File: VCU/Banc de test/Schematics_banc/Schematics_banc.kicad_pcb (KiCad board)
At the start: 2 copper layers, 152.5 x 127 mm, 165 parts, among them IC1 TPS7B8633QDDARQ1, IC2 ATA6561-GBQW-N, IC3 TPS7B8633QDDARQ1, J1 2P Angle 171857-4002, J10 2P Droit 2-11-2022, J11 4P Droit 22-11-2042, J12 DM3AT-SF-PEJM5_40_, J2 2P Droit 2-11-2022, J3 4P Droit 22-11-2042, J4 4P Droit 22-11-2042, J5 6P Droit 22-11-2062, J6 6P Droit 22-11-2062, J7 10-97-7086, J8 10-97-7086, J9 2P Droit 2-11-2022, Q1 MMBF170, Q10 SI2337DS-T1-BE3, Q11 SI2337DS-T1-BE3, Q12 SI2337DS-T1-BE3, Q13 SI2337DS-T1-BE3, Q14 SI2337DS-T1-BE3, Q15 SI2337DS-T1-BE3, Q16 SI2337DS-T1-BE3, Q17 BSS138, Q18 BSS138, Q19 BSS138, Q2 MMBF170, Q20 BSS138, Q3 MMBF170, Q4 MMBF170, Q5 MMBF170, Q6 MMBF170, Q7 MMBF170, Q8 MMBF170, Q9 SI2337DS-T1-BE3

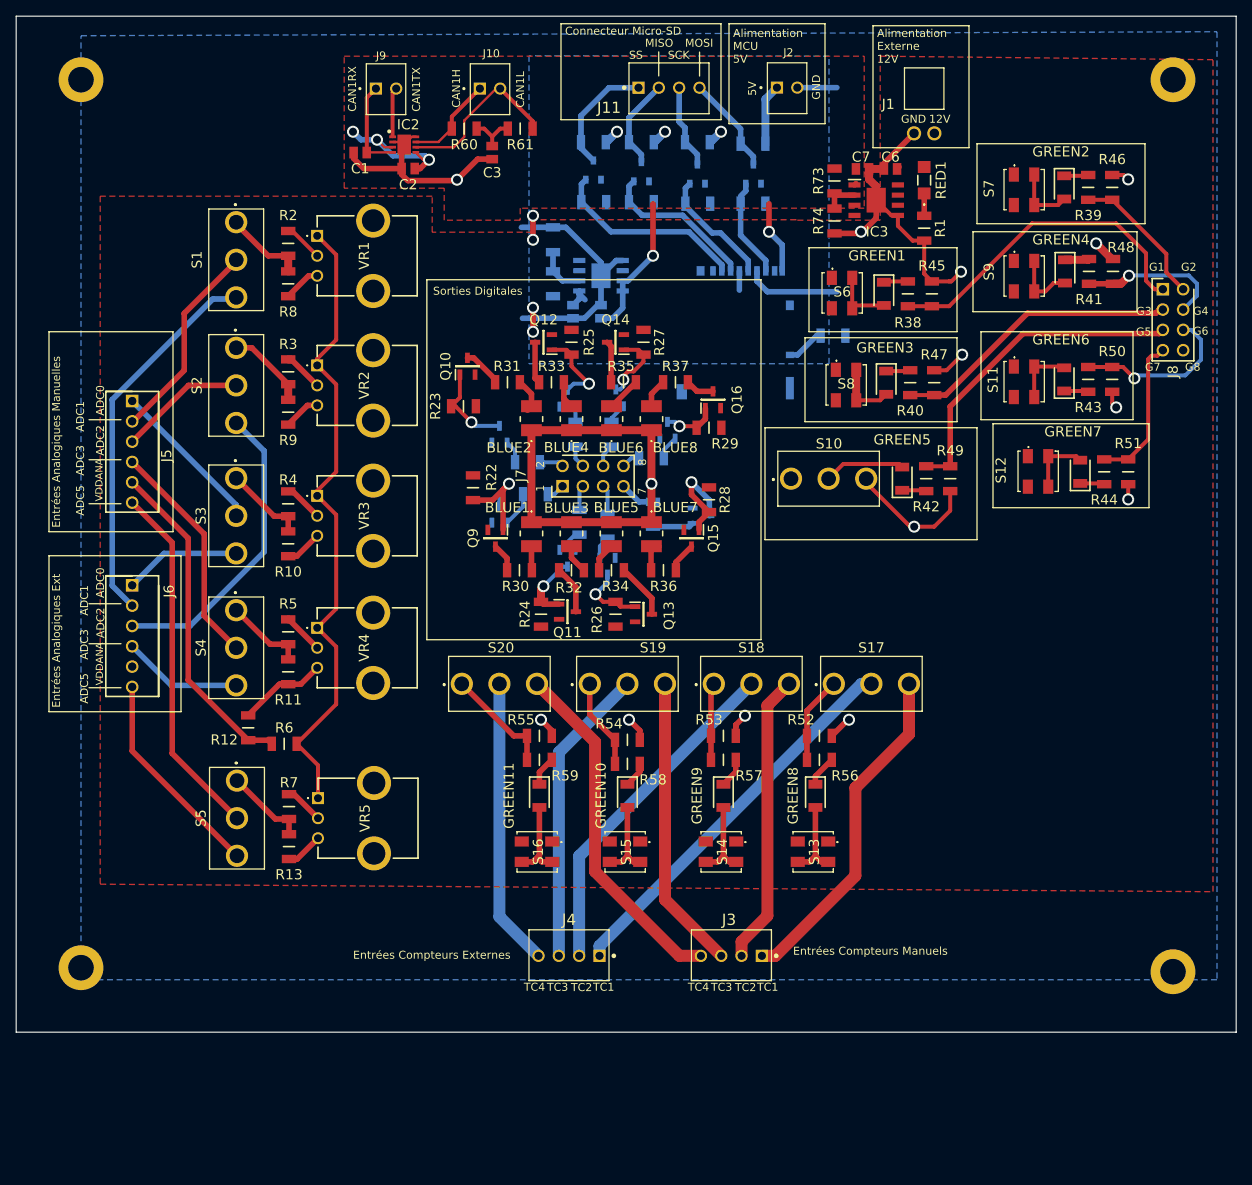
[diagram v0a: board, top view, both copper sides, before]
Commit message: Routage Final
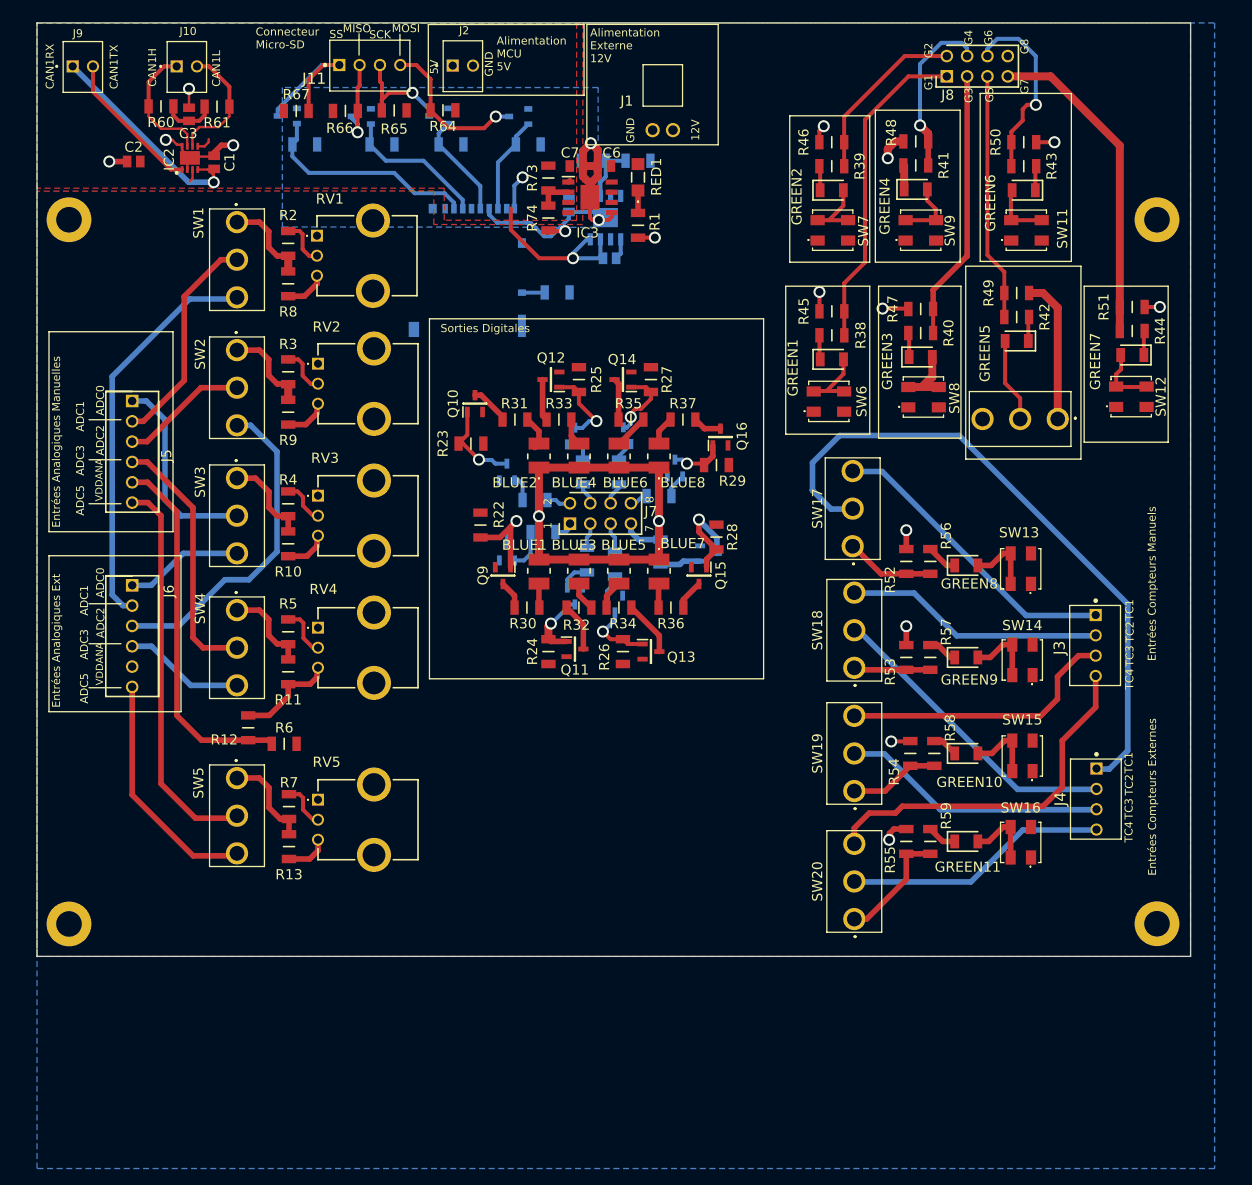
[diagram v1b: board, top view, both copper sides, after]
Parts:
- removed ? (x4): , 
- removed S1, S10, S17, S18, S19, S2, S20, S3, S4, S5: 100SP1T1B4M2QE, Footprints:100SP1T1B4M2QE
- removed S11, S12, S13, S14, S15, S16, S6, S7, S8, S9: 7914J-1-000E, Footprints:7914J1000E
- removed VR1, VR2, VR3, VR4, VR5: PTV09A-4015U-A503, Footprints:PTV09A4015UA503
- added M2: MountingHole_3.2mm_M3_DIN965_Pad, MountingHole:MountingHole_3.2mm_M3_DIN965_Pad, F.Cu at (64.0, 135.0)
- added M2: MountingHole_3.2mm_M3_DIN965_Pad, MountingHole:MountingHole_3.2mm_M3_DIN965_Pad, F.Cu at (64.0, 47.0)
- added M2: MountingHole_3.2mm_M3_DIN965_Pad, MountingHole:MountingHole_3.2mm_M3_DIN965_Pad, F.Cu at (200.0, 135.0)
- added M2: MountingHole_3.2mm_M3_DIN965_Pad, MountingHole:MountingHole_3.2mm_M3_DIN965_Pad, F.Cu at (200.0, 47.0)
- added RV1: R_Potentiometer, Footprints:PTV09A4015UA503, F.Cu at (95.0, 49.0)
- added RV2: R_Potentiometer, Footprints:PTV09A4015UA503, F.Cu at (95.1, 65.0)
- added RV3: R_Potentiometer, Footprints:PTV09A4015UA503, F.Cu at (95.1, 81.5)
- added RV4: R_Potentiometer, Footprints:PTV09A4015UA503, F.Cu at (95.1, 98.0)
- added RV5: R_Potentiometer, Footprints:PTV09A4015UA503, F.Cu at (95.1, 119.5)
- added SW1: 100SP1T1B4M2QE, Footprints:100SP1T1B4M2QE, F.Cu at (85.0, 52.0)
- added SW10: 100SP1T1B4M2QE, Footprints:100SP1T1B4M2QE, F.Cu at (182.9, 71.9)
- added SW11: 7914J-1-000E, Footprints:7914J1000E, F.Cu at (183.4, 48.3)
- added SW12: 7914J-1-000E, Footprints:7914J1000E, F.Cu at (196.5, 69.1)
- added SW13: 7914J-1-000E, Footprints:7914J1000E, F.Cu at (183.0, 90.9)
- added SW14: 7914J-1-000E, Footprints:7914J1000E, F.Cu at (183.2, 102.3)
- added SW15: 7914J-1-000E, Footprints:7914J1000E, F.Cu at (183.2, 114.3)
- added SW16: 7914J-1-000E, Footprints:7914J1000E, F.Cu at (183.0, 125.1)
- added SW17: 100SP1T1B4M2QE, Footprints:100SP1T1B4M2QE, F.Cu at (162.0, 83.1)
- added SW18: 100SP1T1B4M2QE, Footprints:100SP1T1B4M2QE, F.Cu at (162.2, 98.3)
- added SW19: 100SP1T1B4M2QE, Footprints:100SP1T1B4M2QE, F.Cu at (162.2, 113.7)
- added SW2: 100SP1T1B4M2QE, Footprints:100SP1T1B4M2QE, F.Cu at (85.0, 68.0)
- added SW20: 100SP1T1B4M2QE, Footprints:100SP1T1B4M2QE, F.Cu at (162.2, 129.7)
- added SW3: 100SP1T1B4M2QE, Footprints:100SP1T1B4M2QE, F.Cu at (85.0, 84.0)
- added SW4: 100SP1T1B4M2QE, Footprints:100SP1T1B4M2QE, F.Cu at (85.0, 100.5)
- added SW5: 100SP1T1B4M2QE, Footprints:100SP1T1B4M2QE, F.Cu at (85.0, 121.5)
- added SW6: 7914J-1-000E, Footprints:7914J1000E, F.Cu at (158.7, 69.7)
- added SW7: 7914J-1-000E, Footprints:7914J1000E, F.Cu at (159.2, 48.3)
- added SW8: 7914J-1-000E, Footprints:7914J1000E, F.Cu at (170.5, 69.2)
- added SW9: 7914J-1-000E, Footprints:7914J1000E, F.Cu at (170.2, 48.3)
- R64, R65, R66, R67: moved to F.Cu
- moved J4 68.8 mm to (192.4, 119.4), turned to -90 degrees
- moved J3 59.8 mm to (192.3, 100.2), turned to -90 degrees
- moved GREEN11 53.7 mm to (176.2, 124.7), turned to 0 degrees
- moved R55 49.9 mm to (171.7, 124.7), turned to 90 degrees
- moved R59 47.7 mm to (168.7, 124.7), turned to -90 degrees
- moved GREEN10 42.7 mm to (176.2, 113.7), turned to 0 degrees
- moved J2 40.6 mm to (112.0, 27.7)
- moved R64 39.0 mm to (110.7, 33.3)
- moved Q20 38.9 mm to (91.3, 34.0), turned to 180 degrees
- moved R54 38.4 mm to (172.2, 113.7), turned to 90 degrees
- moved C3 38.2 mm to (79.0, 33.8), turned to -90 degrees
- moved R65 38.1 mm to (104.6, 33.3)
- moved R60 38.0 mm to (75.5, 32.8)
- moved J10 38.0 mm to (77.5, 27.8)
- moved J9 38.0 mm to (64.5, 27.8)
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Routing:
- net 12V: track 80.8 -> 0.77 mm
- net GND: track 239.1 -> 195.6 mm, vias 14 -> 20
- net FRWSS_in: track 48.8 -> 82.7 mm
- net 5V: track 59.4 -> 30.3 mm, vias 8 -> 2
- net GPIO4: track 18.9 -> 40.8 mm
- net CAN1RX: track 11.7 -> 27.7 mm, vias 0 -> 1
- net CAN1TX: track 6.14 -> 18.3 mm
- net /Conversion 5V-3.3V/3.3V: track 11.9 -> 0.00 mm, vias 4 -> 0
- net Dry/WetSwitch_st: track 41.0 -> 31.0 mm
- net Net-(GREEN3-A): track 7.87 -> 16.3 mm
- net MOSI_5V: track 12.4 -> 19.8 mm, vias 0 -> 1
- net CAN1L: track 22.2 -> 16.9 mm
- net FBPS: track 19.7 -> 24.8 mm
- net FRWSS_out: track 42.6 -> 37.8 mm
- net LV_BATT: track 41.4 -> 45.9 mm
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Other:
- board size 152.5 x 127 mm -> 144.2 x 116.7 mm
